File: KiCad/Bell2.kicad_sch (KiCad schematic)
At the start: 34 parts, among them J1 USB-C, J2 POWER, J3 Conn_01x10, U1 ESP32-PICO-MINI-02, U2 FT231XQ, U3 ISL89410, U4 ISL89410, U5 LMR16006+FB, U6 AA, U7 QR

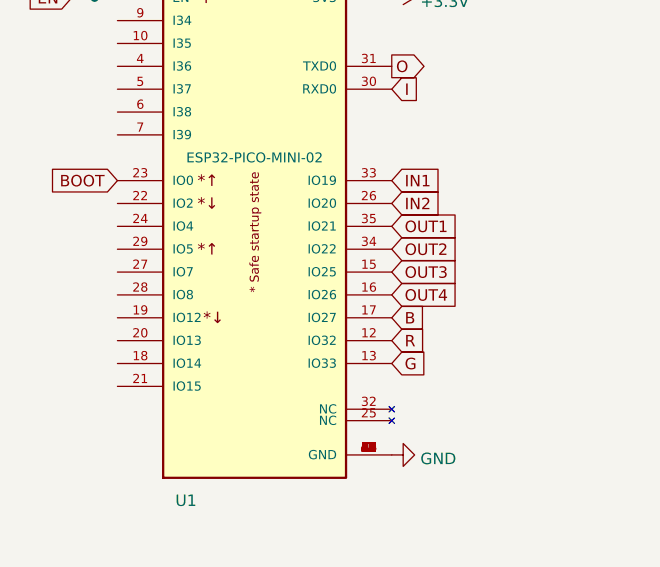
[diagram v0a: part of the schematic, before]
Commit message: Bell2 - tracks and DRC
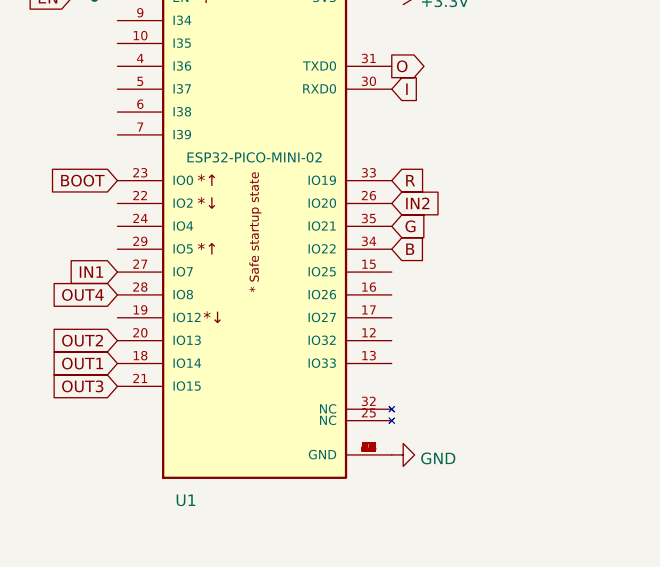
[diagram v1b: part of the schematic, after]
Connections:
- net B: now also U1.34 (IO22); no longer U1.17 (IO27)
- net G: now also U1.35 (IO21); no longer U1.13 (IO33)
- net IN1: now also U1.27 (IO7); no longer U1.33 (IO19)
- net OUT1: now also U1.18 (IO14); no longer U1.35 (IO21)
- net OUT2: now also U1.20 (IO13); no longer U1.34 (IO22)
- net OUT3: now also U1.21 (IO15); no longer U1.15 (IO25)
- net OUT4: now also U1.28 (IO8); no longer U1.16 (IO26)
- net R: now also U1.33 (IO19); no longer U1.12 (IO32)
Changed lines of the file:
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@@
     )
   )
-  (global_label "R" (shape input) (at 66.04 76.2 0) (fields_autoplaced)
-    (effects (font (size 1.27 1.27)) (justify left))
-    (property "Intersheet References" "${INTERSHEET_REFS}" (id 0) (at -2.54 -2.54 0)
+  (global_label "R" (shape input) (at 66.04 58.42 0) (fields_autoplaced)
+    (effects (font (size 1.27 1.27)) (justify left))
+    (property "Intersheet References" "${INTERSHEET_REFS}" (id 0) (at -2.54 -20.32 0)
       (effects (font (size 1.27 1.27)) hide)
     )
@@
     )
   )
-  (global_label "IN1" (shape input) (at 66.04 58.42 0) (fields_autoplaced)
-    (effects (font (size 1.27 1.27)) (justify left))
-    (property "Intersheet References" "${INTERSHEET_REFS}" (id 0) (at -2.54 5.08 0)
+  (global_label "IN1" (shape input) (at 35.56 68.58 180) (fields_autoplaced)
+    (effects (font (size 1.27 1.27)) (justify right))
+    (property "Intersheet References" "${INTERSHEET_REFS}" (id 0) (at 104.14 121.92 0)
       (effects (font (size 1.27 1.27)) hide)
     )
@@
     )
   )
-  (global_label "B" (shape input) (at 66.04 73.66 0) (fields_autoplaced)
-    (effects (font (size 1.27 1.27)) (justify left))
-    (property "Intersheet References" "${INTERSHEET_REFS}" (id 0) (at -2.54 -2.54 0)
+  (global_label "B" (shape input) (at 66.04 66.04 0) (fields_autoplaced)
+    (effects (font (size 1.27 1.27)) (justify left))
+    (property "Intersheet References" "${INTERSHEET_REFS}" (id 0) (at -2.54 -10.16 0)
       (effects (font (size 1.27 1.27)) hide)
     )
@@
     )
   )
-  (global_label "OUT3" (shape input) (at 66.04 68.58 0) (fields_autoplaced)
-    (effects (font (size 1.27 1.27)) (justify left))
-    (property "Intersheet References" "${INTERSHEET_REFS}" (id 0) (at -2.54 -2.54 0)
+  (global_label "OUT3" (shape input) (at 35.56 81.28 180) (fields_autoplaced)
+    (effects (font (size 1.27 1.27)) (justify right))
+    (property "Intersheet References" "${INTERSHEET_REFS}" (id 0) (at 104.14 152.4 0)
       (effects (font (size 1.27 1.27)) hide)
     )
@@
     )
   )
-  (global_label "OUT2" (shape input) (at 66.04 66.04 0) (fields_autoplaced)
-    (effects (font (size 1.27 1.27)) (justify left))
-    (property "Intersheet References" "${INTERSHEET_REFS}" (id 0) (at -2.54 -2.54 0)
+  (global_label "OUT2" (shape input) (at 35.56 76.2 180) (fields_autoplaced)
+    (effects (font (size 1.27 1.27)) (justify right))
+    (property "Intersheet References" "${INTERSHEET_REFS}" (id 0) (at 104.14 144.78 0)
       (effects (font (size 1.27 1.27)) hide)
     )
@@
     )
   )
-  (global_label "G" (shape input) (at 66.04 78.74 0) (fields_autoplaced)
-    (effects (font (size 1.27 1.27)) (justify left))
-    (property "Intersheet References" "${INTERSHEET_REFS}" (id 0) (at -2.54 -2.54 0)
-      (effects (font (size 1.27 1.27)) hide)
-    )
-  )
-  (global_label "OUT1" (shape input) (at 66.04 63.5 0) (fields_autoplaced)
-    (effects (font (size 1.27 1.27)) (justify left))
-    (property "Intersheet References" "${INTERSHEET_REFS}" (id 0) (at -2.54 -2.54 0)
+  (global_label "G" (shape input) (at 66.04 63.5 0) (fields_autoplaced)
+    (effects (font (size 1.27 1.27)) (justify left))
+    (property "Intersheet References" "${INTERSHEET_REFS}" (id 0) (at -2.54 -17.78 0)
+      (effects (font (size 1.27 1.27)) hide)
+    )
+  )
+  (global_label "OUT1" (shape input) (at 35.56 78.74 180) (fields_autoplaced)
+    (effects (font (size 1.27 1.27)) (justify right))
+    (property "Intersheet References" "${INTERSHEET_REFS}" (id 0) (at 104.14 144.78 0)
       (effects (font (size 1.27 1.27)) hide)
     )
@@
     )
   )
-  (global_label "OUT4" (shape input) (at 66.04 71.12 0) (fields_autoplaced)
-    (effects (font (size 1.27 1.27)) (justify left))
-    (property "Intersheet References" "${INTERSHEET_REFS}" (id 0) (at -2.54 -2.54 0)
-      (effects (font (size 1.27 1.27)) hide)
-    )
+  (global_label "OUT4" (shape input) (at 35.56 71.12 180) (fields_autoplaced)
+    (effects (font (size 1.27 1.27)) (justify right))
+    (property "Intersheet References" "${INTERSHEET_REFS}" (id 0) (at 104.14 144.78 0)
+      (effects (font (size 1.27 1.27)) hide)
+    )
